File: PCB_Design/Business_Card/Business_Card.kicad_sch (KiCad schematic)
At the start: 18 parts, among them J1 1-14in IPS ST7789V Display, SW1 Main Power, SW2 SW_Push, SW3 SW_Push, SW4 SW_Push, SW5 SW_Push, U1 XIAO nRF52840

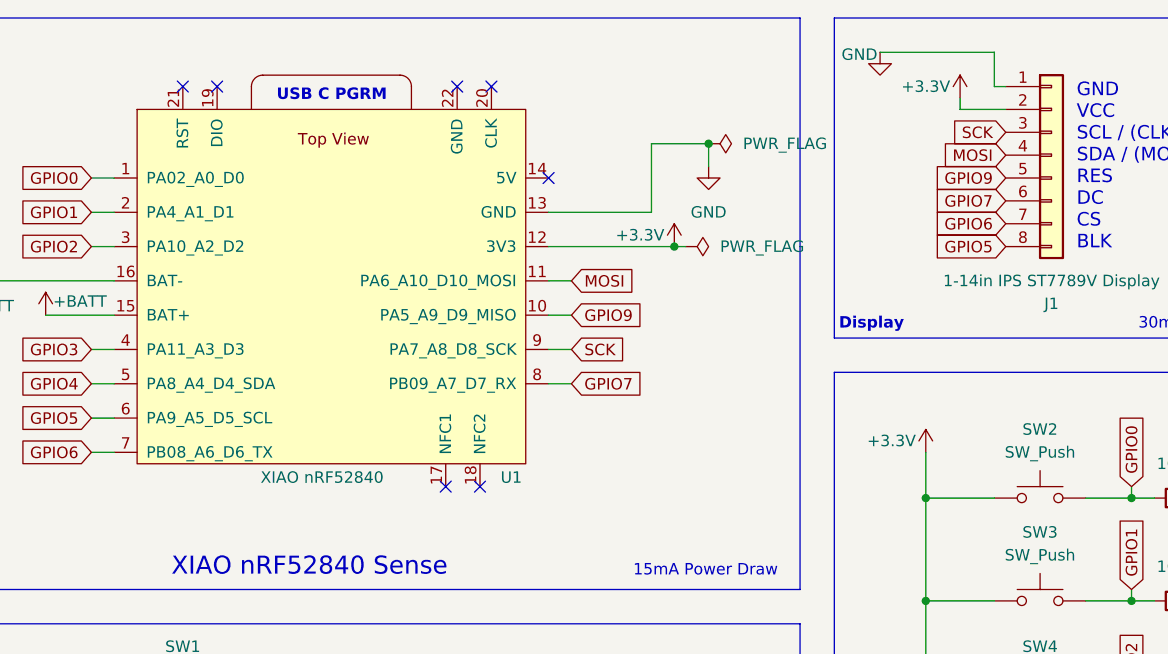
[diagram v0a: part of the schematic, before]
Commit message: PCB Schematic and Layout Updates
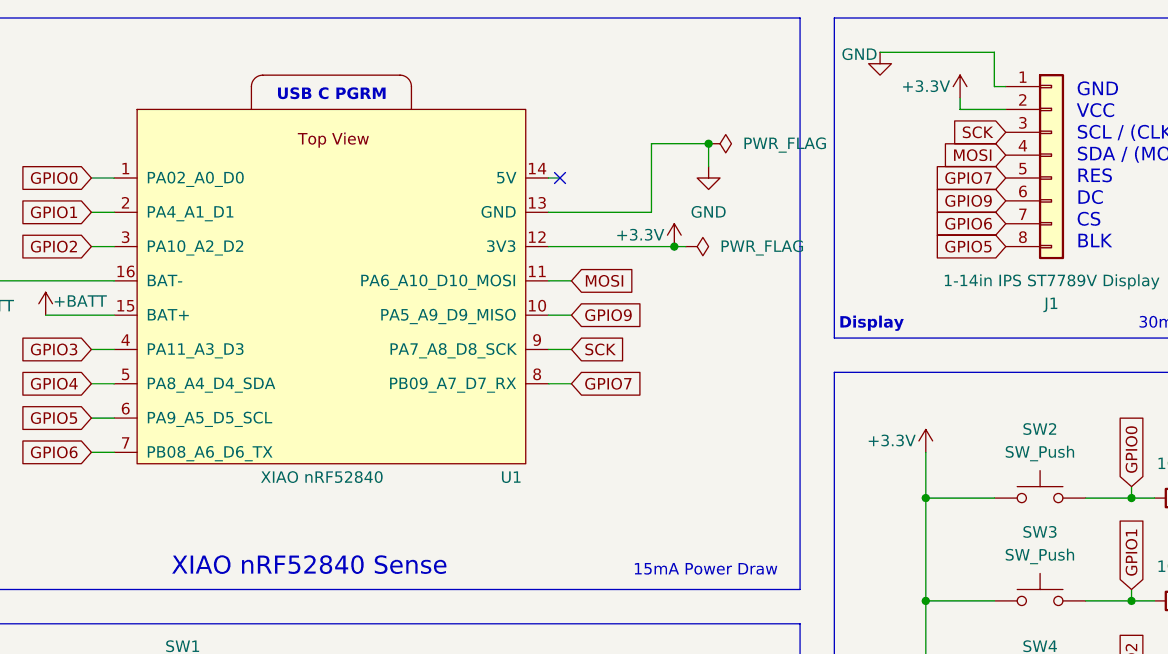
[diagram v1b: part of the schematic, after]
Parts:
- J1: footprint Connector_PinHeader_2.54mm:PinHeader_1x08_P2.54mm_Vertical -> GanlathLib:1-14in_IPS_ST7789V_Display
- SW1: footprint Connector_PinHeader_2.54mm:PinHeader_1x02_P2.54mm_Vertical -> GanlathLib:BlankPin_1x02_P2.54mm
- U1: footprint GanlathLib:XIAO-nRF52840-SMD -> GanlathLib:XIAO-nRF52840-SMD_Revised; symbol GanlathLib:XIAO nRF52840 -> GanlathLib:XIAO nRF52840_Revised
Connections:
- net GPIO7: now also J1.5 (Pin_5); no longer J1.6 (Pin_6)
- net GPIO9: now also J1.6 (Pin_6); no longer J1.5 (Pin_5)
- no-connect marks 7 -> 1
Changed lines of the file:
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@@
 	)
 	(no_connect
-		(at 92.71 33.02)
-	)
-	(no_connect
-		(at 55.88 22.86)
-	)
-	(no_connect
-		(at 52.07 22.86)
-	)
-	(no_connect
-		(at 86.36 22.86)
-	)
-	(no_connect
-		(at 81.28 67.31)
-	)
-	(no_connect
-		(at 82.55 22.86)
-	)
-	(no_connect
-		(at 85.09 67.31)
+		(at 93.98 33.02)
 	)
 	(wire
@@
 		(pts
 			(xy 142.24 106.68) (xy 134.62 106.68)
+		)
+		(stroke
+			(width 0)
+			(type default)
+		)
+	)
+	(wire
+		(pts
+			(xy 93.98 33.02) (xy 92.71 33.02)
 		)
 		(stroke
@@
 	(global_label "GPIO9"
 		(shape input)
-		(at 95.25 48.26 0)
+		(at 143.51 35.56 180)
 		(fields_autoplaced yes)
 		(effects
@@
 				(size 1.27 1.27)
 			)
+			(justify right)
+		)
+		(property "Intersheetrefs" "${INTERSHEET_REFS}"
+			(at 134.7449 35.56 0)
+			(effects
+				(font
+					(size 1.27 1.27)
+				)
+				(justify right)
+				(hide yes)
+			)
+		)
+	)
+	(global_label "GPIO9"
+		(shape input)
+		(at 95.25 48.26 0)
+		(fields_autoplaced yes)
+		(effects
+			(font
+				(size 1.27 1.27)
+			)
 			(justify left)
 		)
@@
 		)
 	)
+	(global_label "GPIO7"
+		(shape input)
+		(at 143.51 33.02 180)
+		(fields_autoplaced yes)
+		(effects
+			(font
+				(size 1.27 1.27)
+			)
+			(justify right)
+		)
+		(property "Intersheetrefs" "${INTERSHEET_REFS}"
+			(at 134.7449 33.02 0)
+			(effects
+				(font
+					(size 1.27 1.27)
+				)
+				(justify right)
+				(hide yes)
+			)
+		)
+	)
 	(global_label "GPIO5"
 		(shape input)
@@
 		)
 	)
-	(global_label "GPIO7"
+	(global_label "GPIO2"
 		(shape input)
-		(at 143.51 35.56 180)
+		(at 157.48 91.44 90)
 		(fields_autoplaced yes)
 		(effects
@@
 				(size 1.27 1.27)
 			)
-			(justify right)
+			(justify left)
 		)
 		(property "Intersheetrefs" "${INTERSHEET_REFS}"
-			(at 134.7449 35.56 0)
-			(effects
-				(font
-					(size 1.27 1.27)
-				)
-				(justify right)
-				(hide yes)
-			)
-		)
-	)
-	(global_label "GPIO2"
+			(at 157.48 82.6749 90)
+			(effects
+				(font
+					(size 1.27 1.27)
+				)
+				(justify left)
+				(hide yes)
+			)
+		)
+	)
+	(global_label "GPIO4"
 		(shape input)
-		(at 157.48 91.44 90)
+		(at 41.91 55.88 180)
 		(fields_autoplaced yes)
 		(effects
@@
 				(size 1.27 1.27)
 			)
-			(justify left)
-		)
-		(property "Intersheetrefs" "${INTERSHEET_REFS}"
-			(at 157.48 82.6749 90)
-			(effects
-				(font
-					(size 1.27 1.27)
-				)
-				(justify left)
-				(hide yes)
-			)
-		)
-	)
-	(global_label "GPIO4"
-		(shape input)
-		(at 41.91 55.88 180)
-		(fields_autoplaced yes)
-		(effects
-			(font
-				(size 1.27 1.27)
-			)
 			(justify right)
 		)
 		(property "Intersheetrefs" "${INTERSHEET_REFS}"
 			(at 33.1449 55.88 0)
-			(effects
-				(font
-					(size 1.27 1.27)
-				)
-				(justify right)
-				(hide yes)
-			)
-		)
-	)
-	(global_label "GPIO9"
-		(shape input)
-		(at 143.51 33.02 180)
-		(fields_autoplaced yes)
-		(effects
-			(font
-				(size 1.27 1.27)
-			)
-			(justify right)
-		)
-		(property "Intersheetrefs" "${INTERSHEET_REFS}"
-			(at 134.7449 33.02 0)
 			(effects
 				(font
@@
 			)
 		)
-		(property "Footprint" "Connector_PinHeader_2.54mm:PinHeader_1x02_P2.54mm_Vertical"
+		(property "Footprint" "GanlathLib:BlankPin_1x02_P2.54mm"
 			(at 52.07 91.44 0)
 			(effects
@@
 			)
 		)
-		(property "Footprint" "Connector_PinHeader_2.54mm:PinHeader_1x08_P2.54mm_Vertical"
+		(property "Footprint" "GanlathLib:1-14in_IPS_ST7789V_Display"
 			(at 148.59 30.48 0)
 			(effects
@@
 	)
 	(symbol
-		(lib_id "GanlathLib:XIAO nRF52840")
+		(lib_id "GanlathLib:XIAO nRF52840_Revised")
 		(at 68.58 43.18 0)
 		(unit 1)
@@
 			)
 		)
-		(property "Footprint" "GanlathLib:XIAO-nRF52840-SMD"
+		(property "Footprint" "GanlathLib:XIAO-nRF52840-SMD_Revised"
 			(at 60.452 70.612 0)
 			(effects
@@
 		(pin "6"
 		)
-		(pin "20"
-		)
-		(pin "22"
-		)
 		(pin "10"
 		)
-		(pin "21"
-		)
 		(pin "13"
 		)
@@
 		(pin "1"
 		)
-		(pin "19"
-		)
 		(pin "15"
 		)
@@
 		(pin "3"
 		)
-		(pin "18"
-		)
 		(pin "2"
 		)
@@
 		(pin "5"
 		)
-		(pin "17"
-		)
 		(instances

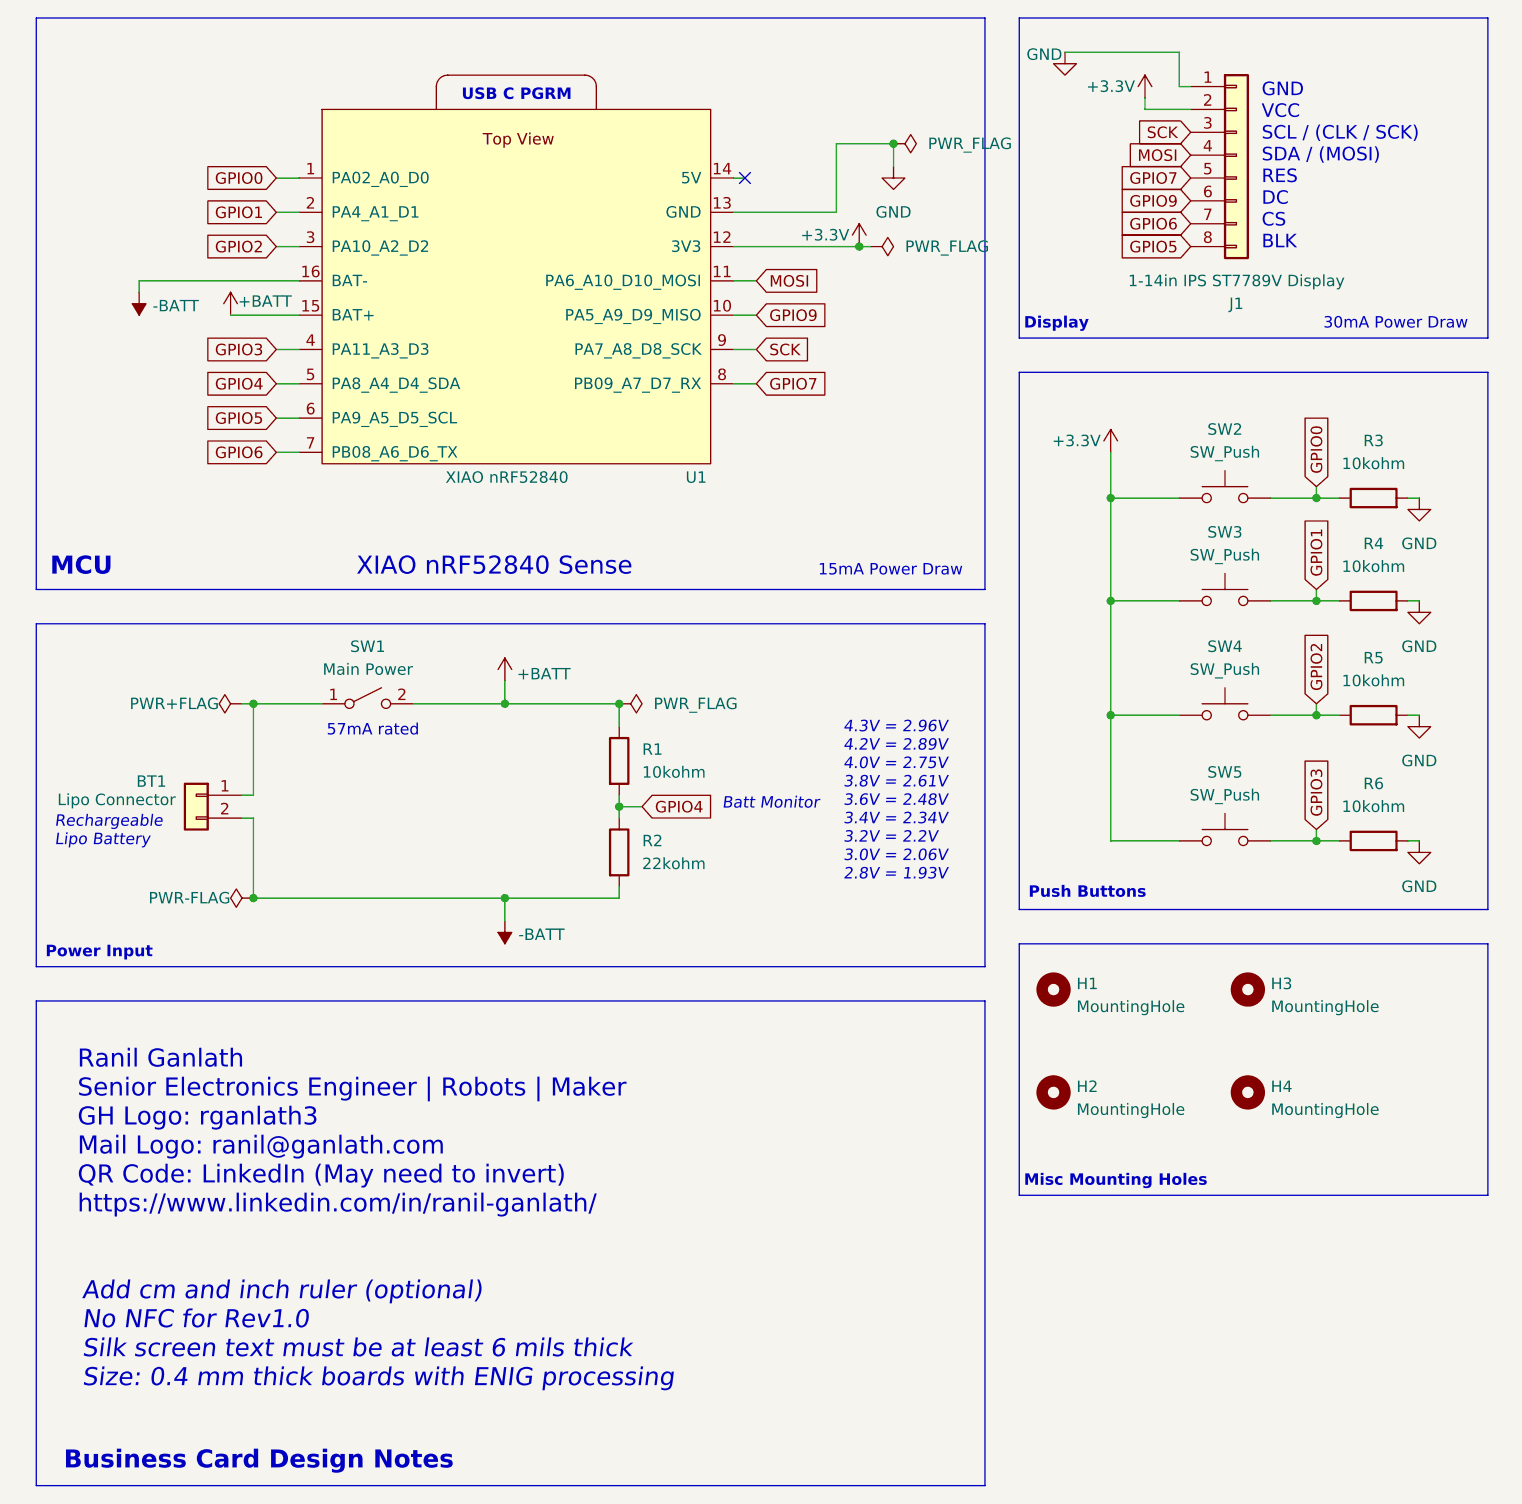
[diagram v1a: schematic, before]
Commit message: PCB Revisions
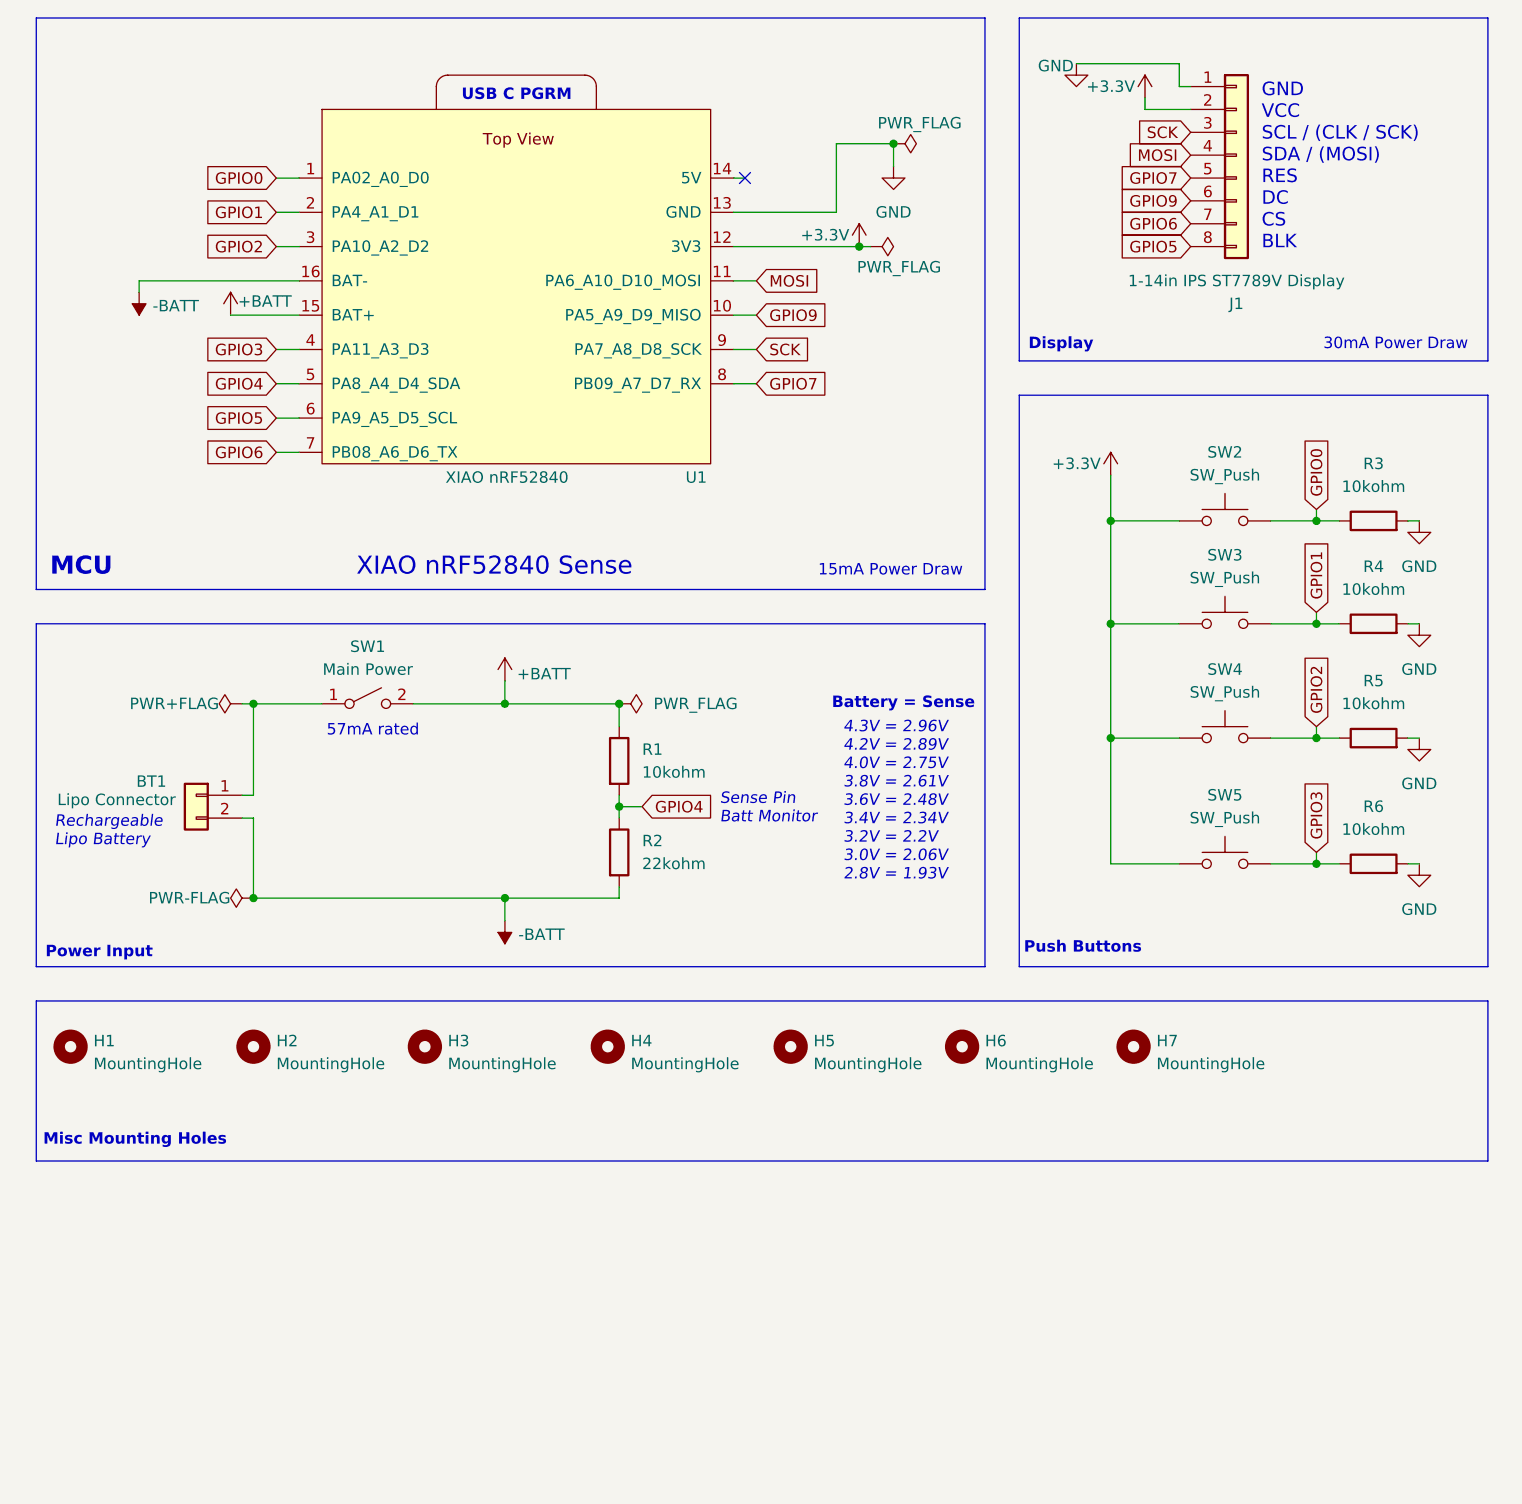
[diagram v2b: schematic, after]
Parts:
- added H5, H7: MountingHole, GanlathLib:MountingHole_3.7mm_Core, symbol Mechanical:MountingHole
- added H6: MountingHole, GanlathLib:MountingHole_3.7mm_Lanyard_Core, symbol Mechanical:MountingHole
- BT1: footprint Connector_JST:JST_XH_B2B-XH-A_1x02_P2.50mm_Vertical -> Connector_PinHeader_2.00mm:PinHeader_2x01_P2.00mm_Vertical_SMD
- H1, H2, H3, H4: footprint MountingHole:MountingHole_3mm -> MountingHole:MountingHole_2.5mm_Pad_TopOnly
- SW1: footprint GanlathLib:BlankPin_1x02_P2.54mm -> Connector_PinHeader_2.00mm:PinHeader_2x01_P2.00mm_Vertical_SMD
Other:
- note added: "Battery = Sense"
- note added: "Sense Pin Batt Monitor"
- note removed: "Add cm and inch ruler (optional) No NFC for Rev1.0 Silk screen text must be at least 6 mils thick Size: 0.4 mm thick boards with ENIG processing"
- note removed: "Batt Monitor"
- note removed: "Business Card Design Notes"
- note removed: "Ranil Ganlath Senior Electronics Engineer | Robots | Maker GH Logo: rganlath3 Mail Logo: ranil@ganlath.com QR Code: LinkedIn (May need to invert) https://www.linkedin.com/in/ranil-ganlath/"
- moved on the sheet: H1, H2, H3, H4, R3, R4, R5, R6, SW2, SW3, SW4, SW5
